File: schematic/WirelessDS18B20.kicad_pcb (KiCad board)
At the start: 2 copper layers, 25.4 x 26.3 mm, 9 parts, among them P1 1-Wire Bus, Q1 2N7002, Q2 2N7002, U1 WeMos_mini, U2 AMS1117-3.3

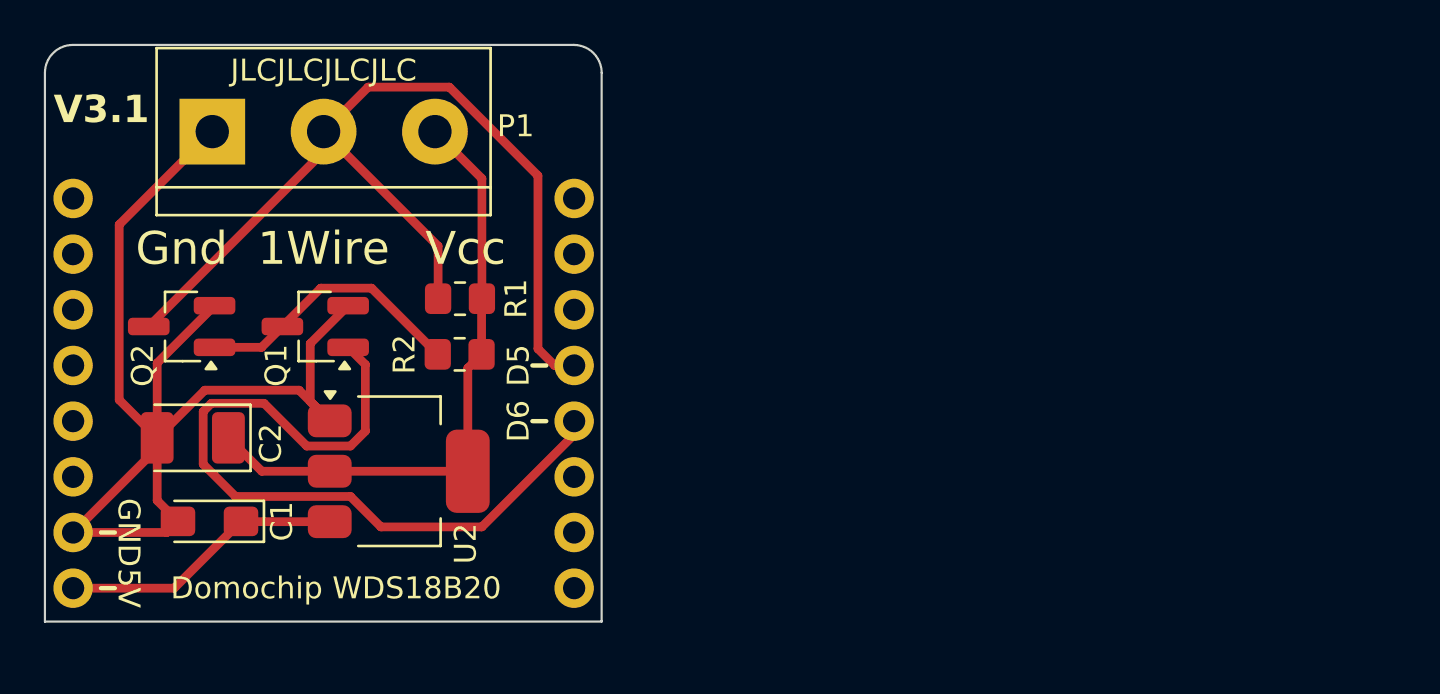
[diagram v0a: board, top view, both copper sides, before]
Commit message: Update schematic and PCB
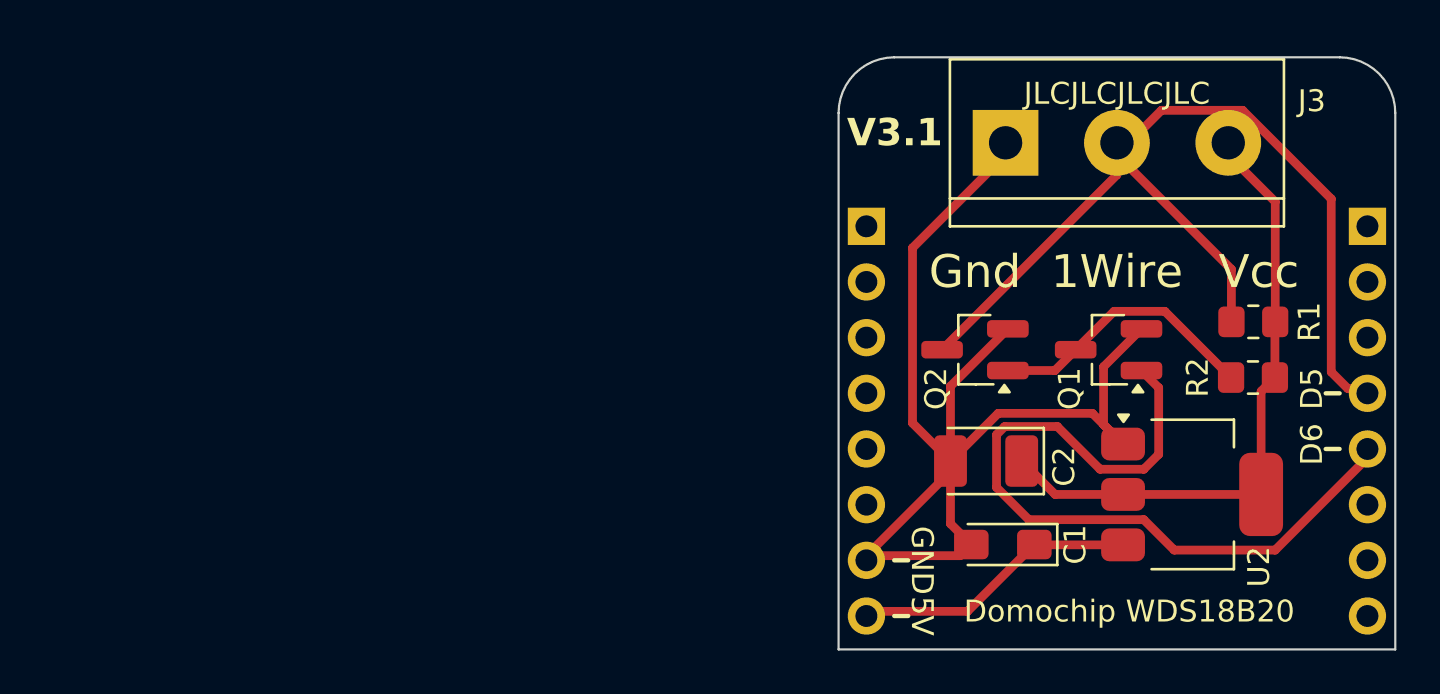
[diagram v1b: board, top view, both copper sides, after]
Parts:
- removed P1: 1-Wire Bus, TerminalBlock:TerminalBlock_bornier-3_P5.08mm
- removed U1: WeMos_mini, wemos_d1_mini:wemos-d1-mini-DIL-only
- added J1: WeMos_mini_Hat_Left, wemos_d1_mini:WeMos_D1_mini_Hat_Left, B.Cu at (61.0, 33.0)
- added J2: WeMos_mini_Hat_Right, wemos_d1_mini:WeMos_D1_mini_Hat_Right, B.Cu at (83.8, 33.0)
- added J3: 1-Wire Bus, TerminalBlock:TerminalBlock_bornier-3_P5.08mm, F.Cu at (67.3, 29.2)
- moved C1 36.2 mm to (67.2, 47.5)
- moved C2 36.2 mm to (66.4, 43.7)
- moved Q1 36.2 mm to (72.0, 38.6)
- moved R1 36.2 mm to (78.6, 37.4)
- moved U2 36.2 mm to (75.8, 45.3)
- moved Q2 36.2 mm to (65.9, 38.6)
- moved R2 36.2 mm to (78.6, 39.9)
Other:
- board size 25.4 x 26.3 mm -> 25.4 x 27 mm
